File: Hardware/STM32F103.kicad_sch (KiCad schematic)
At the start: 18 parts, among them J2 Conn_02x03_Odd_Even, J3 Conn_02x04_Counter_Clockwise, SW3 SW_Push, U5 MCU_STM32F103C8Tx, Y1 8Mhz

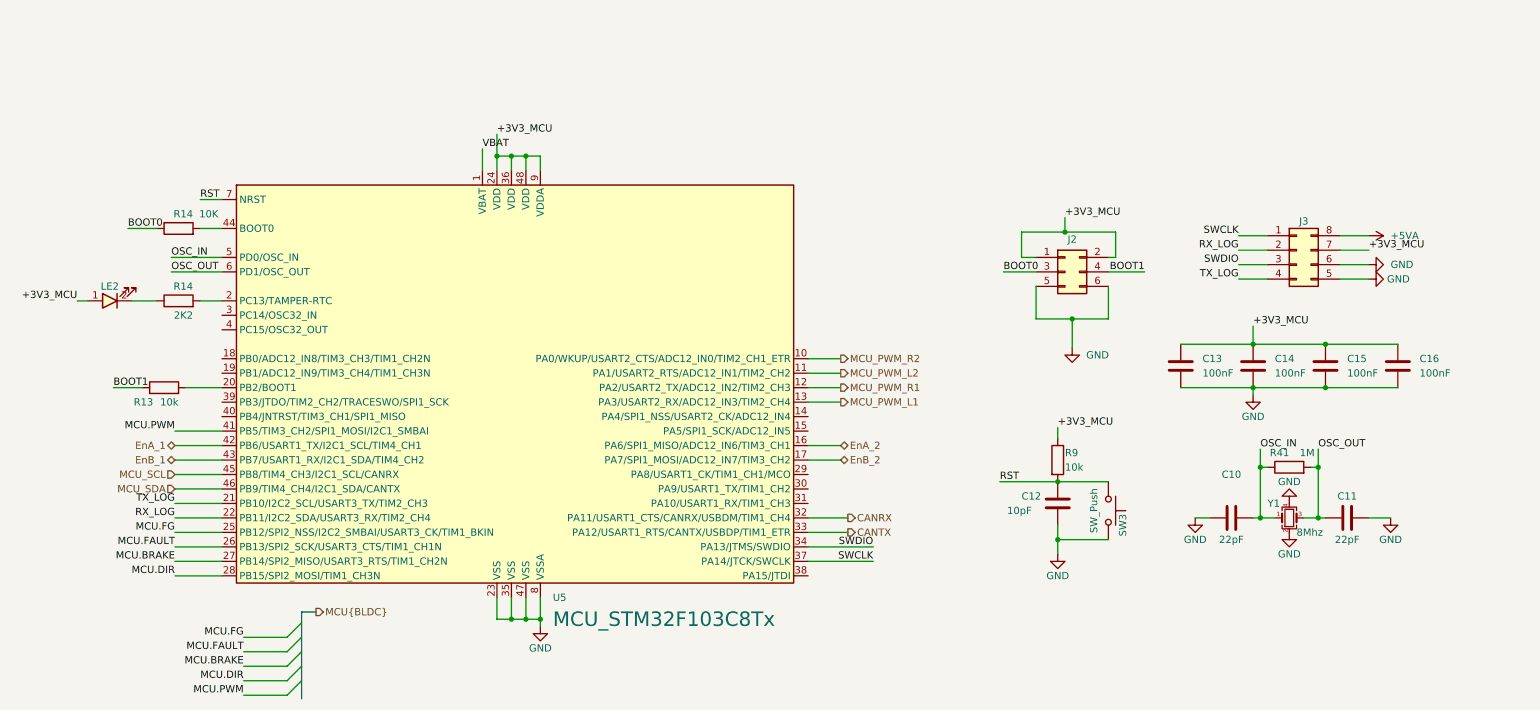
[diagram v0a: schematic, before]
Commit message: Add PCB
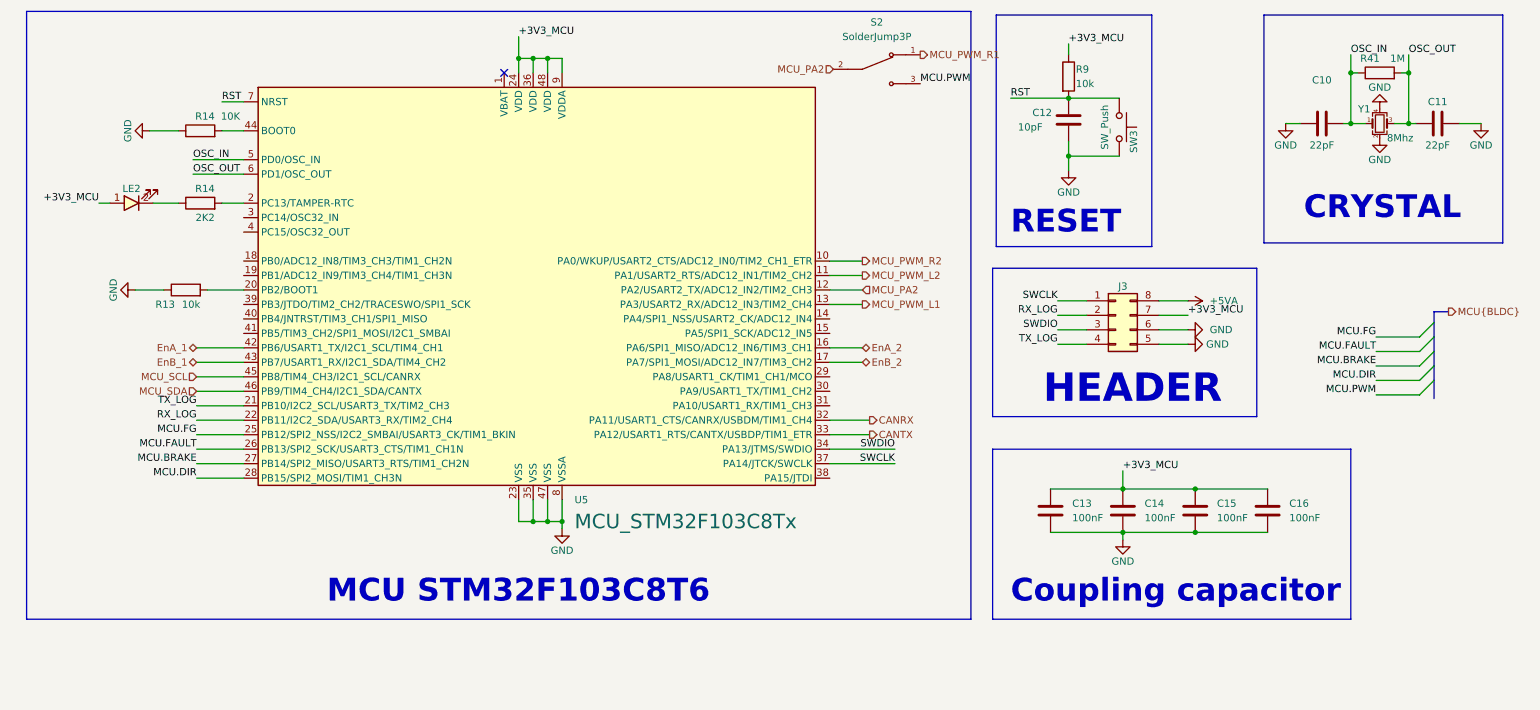
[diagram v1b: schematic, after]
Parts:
- removed J2: Conn_02x03_Odd_Even, Connector_PinHeader_2.54mm:PinHeader_2x03_P2.54mm_Vertical, symbol Connector_Generic:Conn_02x03_Odd_Even
- added S2: SolderJump3P, Jumper:SolderJumper-3_P1.3mm_Open_RoundedPad1.0x1.5mm_NumberLabels, symbol IVS_SYMBOLS:EG1206
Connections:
- net BOOT0 is gone; now on net GND: R14.1
- net BOOT1 is gone; now on net GND: R13.1
- net MCU.PWM: now also S2.3; no longer U5.41 (PB5/TIM3_CH2/SPI1_MOSI/I2C1_SMBAI)
- net MCU_PWM_R1: now also S2.1; no longer U5.12 (PA2/USART2_TX/ADC12_IN2/TIM2_CH3)
- net VBAT: no longer names the net of U5.1 (VBAT)
- new net MCU_PA2: S2.2, U5.12 (PA2/USART2_TX/ADC12_IN2/TIM2_CH3)
- no-connect marks 0 -> 1
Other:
- note added: "CRYSTAL"
- note added: "Coupling capacitor"
- note added: "HEADER"
- note added: "MCU STM32F103C8T6"
- note added: "RESET"
- moved on the sheet: C10, C11, C12, C13, C14, C15, C16, J3, LE2, R13, R14, R41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
